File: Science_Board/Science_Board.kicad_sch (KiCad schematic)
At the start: 25 parts, among them J1 Conn_01x02, J10 Conn_01x02, J11 Conn_01x03, J12 Conn_01x03, J13 Conn_01x03, J14 Conn_01x03, J15 Conn_01x03, J16 Conn_01x03, J17 Conn_01x03, J18 Conn_01x03, J19 Conn_01x02, J20 Molex_Megafit_02, J5 Conn_01x02, J6 Conn_01x04, J7 Conn_01x03, J8 Conn_01x03, J9 Conn_01x02, U5 PCA9685BS

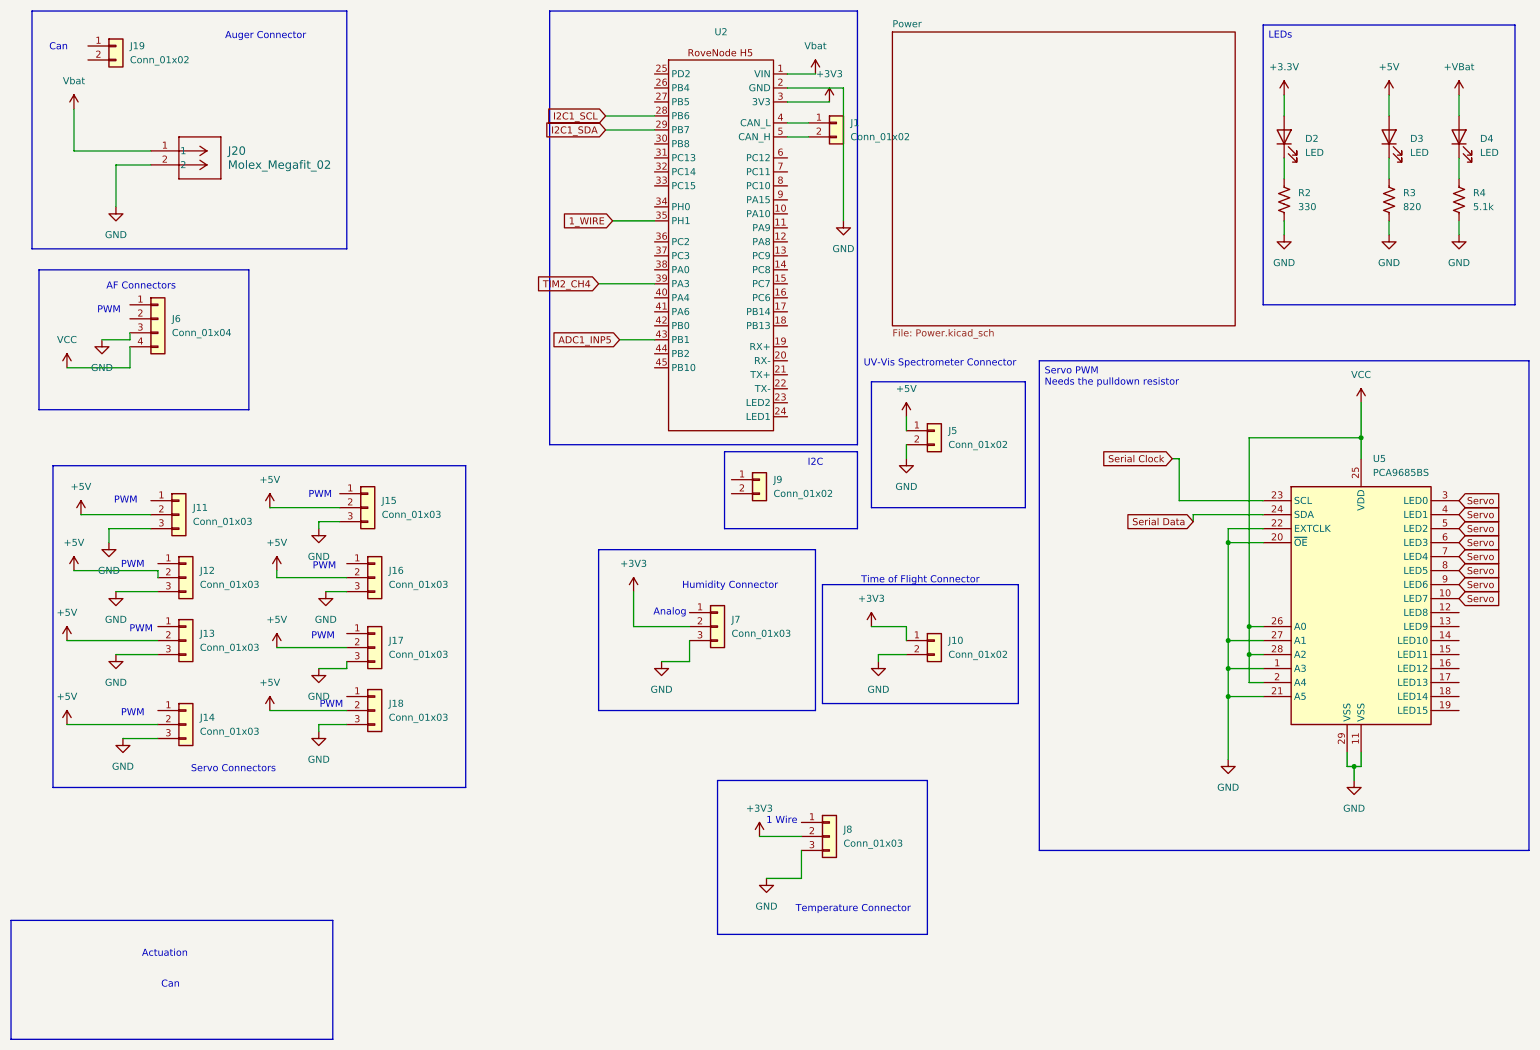
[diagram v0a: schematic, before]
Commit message: Hooked up a lot of connections
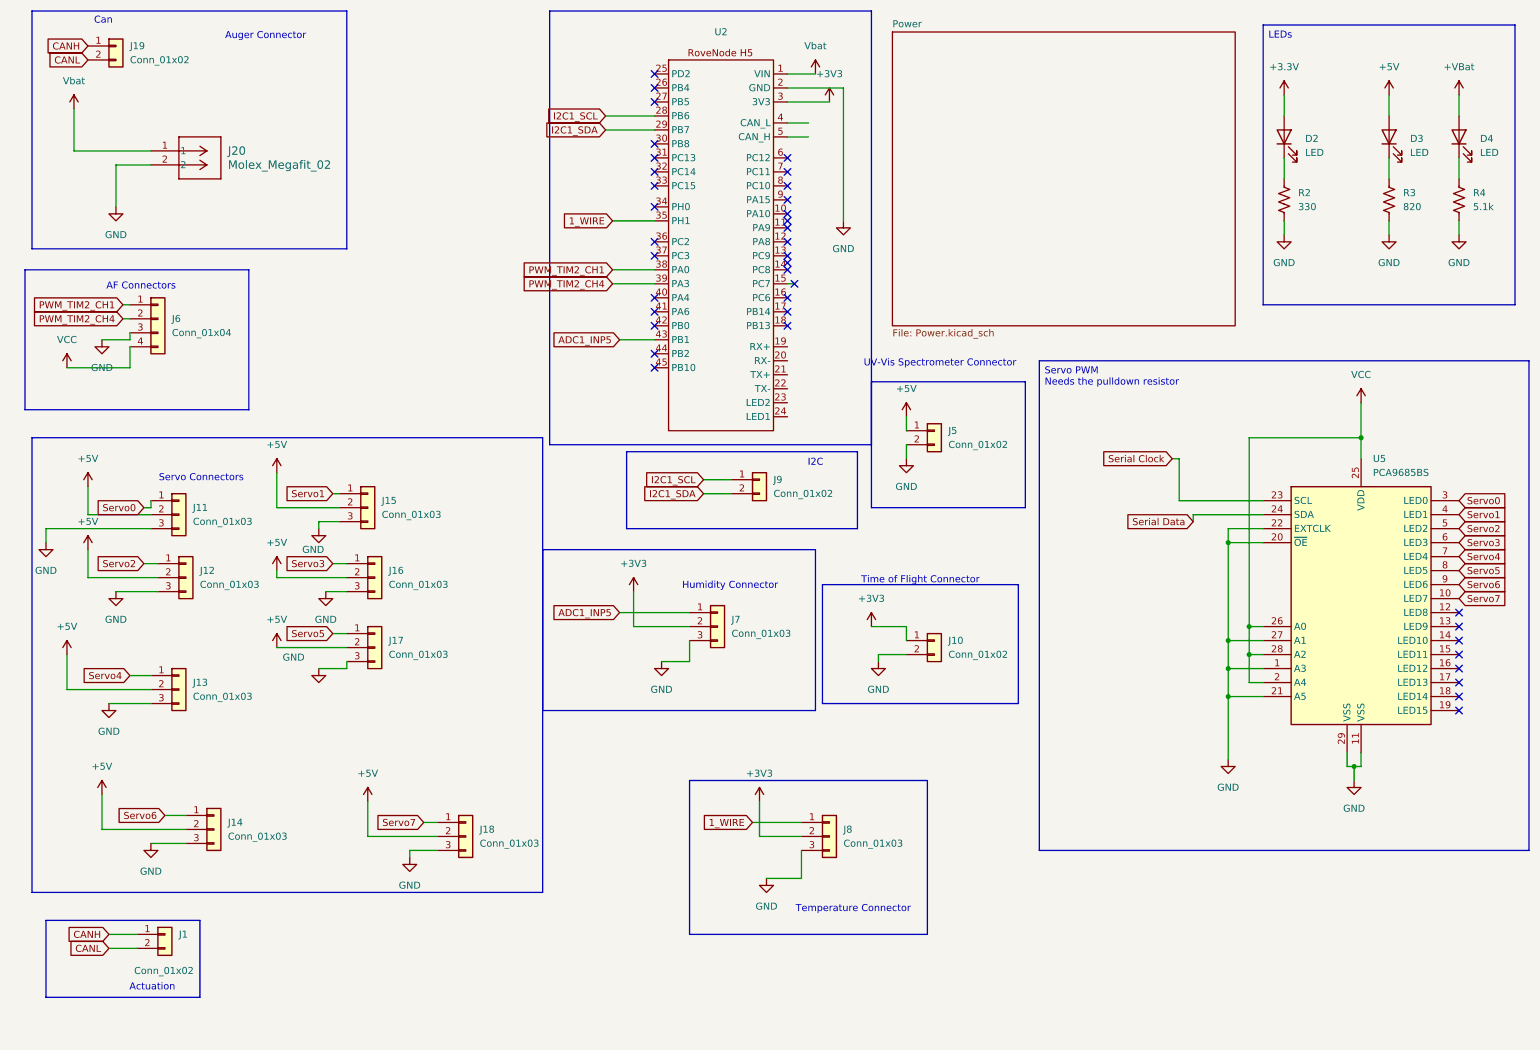
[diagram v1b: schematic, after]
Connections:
- net TIM2_CH4 is gone; now on net PWM_TIM2_CH4: U2.39 (PA3)
- net 1_WIRE: now also J8.1 (Pin_1)
- net ADC1_INP5: now also J7.1 (Pin_1)
- net I2C1_SCL: now also J9.1 (Pin_1)
- net I2C1_SDA: now also J9.2 (Pin_2)
- net Servo2: now reaches J12.1 (Pin_1)
- net Servo2: now also U5.5 (LED2)
- net Servo1: now reaches J15.1 (Pin_1)
- net Servo1: now also U5.4 (LED1)
- net CANH: now reaches J19.1 (Pin_1)
- net CANH: now also J1.1 (Pin_1)
- net CANL: now reaches J19.2 (Pin_2)
- net CANL: now also J1.2 (Pin_2)
- net Servo4: now reaches J13.1 (Pin_1)
- net Servo4: now also U5.7 (LED4)
- net Servo5: now reaches J17.1 (Pin_1)
- net Servo5: now also U5.8 (LED5)
- net PWM_TIM2_CH1: now reaches J6.1 (Pin_1)
- net PWM_TIM2_CH1: now also U2.38 (PA0)
- net PWM_TIM2_CH4: now reaches J6.2 (Pin_2)
- net Servo3: now reaches J16.1 (Pin_1)
- net Servo3: now also U5.6 (LED3)
- net Servo0: now reaches J11.1 (Pin_1)
- net Servo0: now also U5.3 (LED0)
- net at U2.4 (CAN_L): no longer J1.1 (Pin_1)
- net at U2.5 (CAN_H): no longer J1.2 (Pin_2)
- net Servo6: now reaches J14.1 (Pin_1)
- net Servo6: now also U5.9 (LED6)
- net Servo7: now reaches J18.1 (Pin_1)
- net Servo7: now also U5.10 (LED7)
- removed net Servo: U5.10 (LED7), U5.3 (LED0), U5.4 (LED1), U5.5 (LED2), U5.6 (LED3), U5.7 (LED4), U5.8 (LED5), U5.9 (LED6)
- no-connect marks 0 -> 38
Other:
- note removed: "1 Wire"
- note removed: "Analog"
- note removed: "PWM"
- moved on the sheet: J13, J14, J18
